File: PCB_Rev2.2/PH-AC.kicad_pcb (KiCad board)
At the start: 2 copper layers, 200 x 100 mm, 51 parts, among them J1 USB_C_Receptacle_USB2.0_16P, J2 Conn_01x03, SW1 SW_Push, SW10 SW_Push, SW2 RotaryEncoder_Switch_MP, SW3 RotaryEncoder_Switch_MP, SW4 SW_Push, SW5 SW_Push, SW6 SW_Push, SW7 SW_Push, SW8 SW_Push, SW9 SW_Push, U1 RP2040, U2 AMS1117-3.3, U3 W25Q16JVSS, Y1 Crystal_GND24

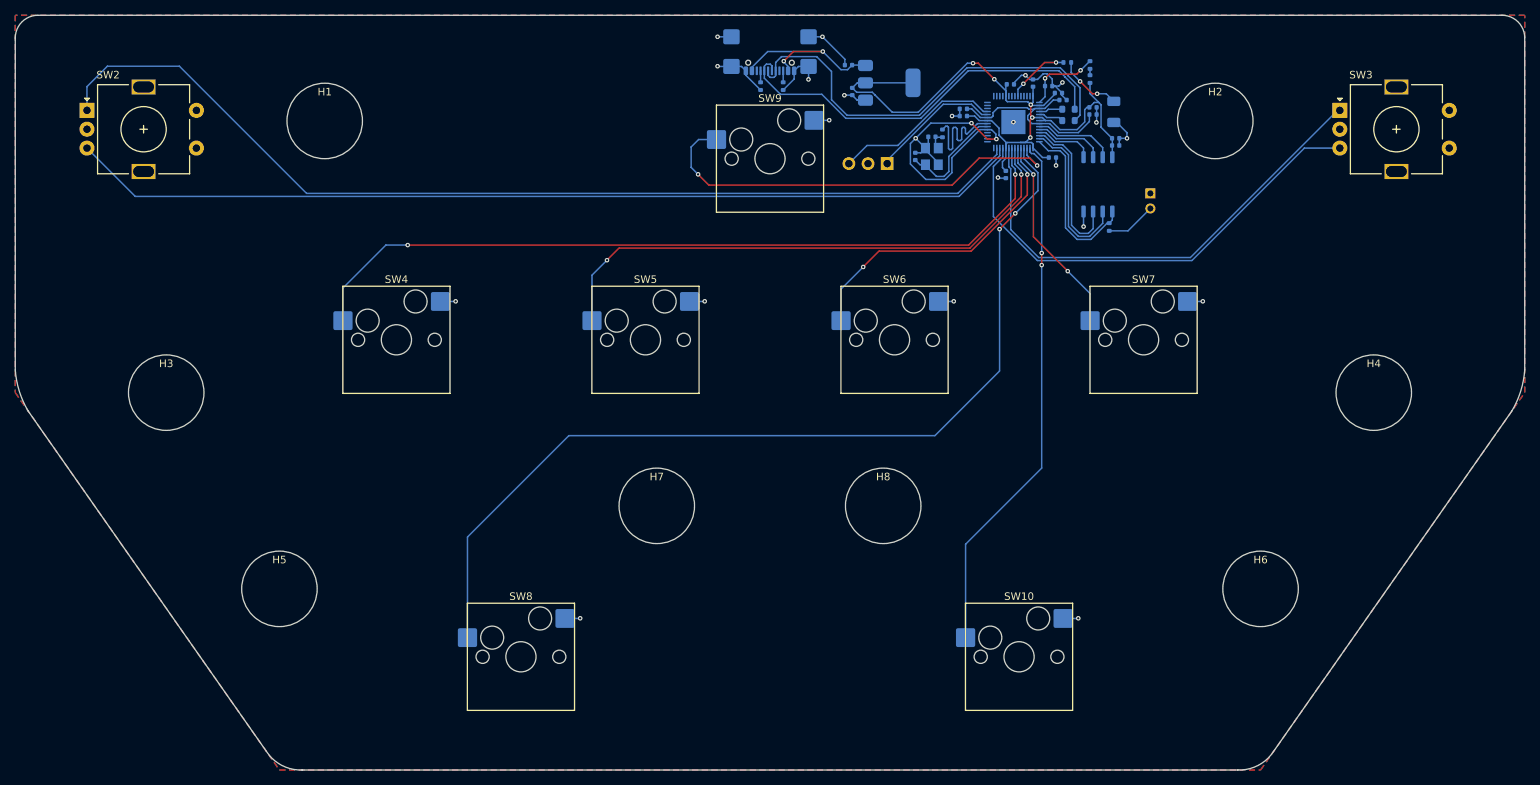
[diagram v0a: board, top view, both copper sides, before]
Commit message: Redesign
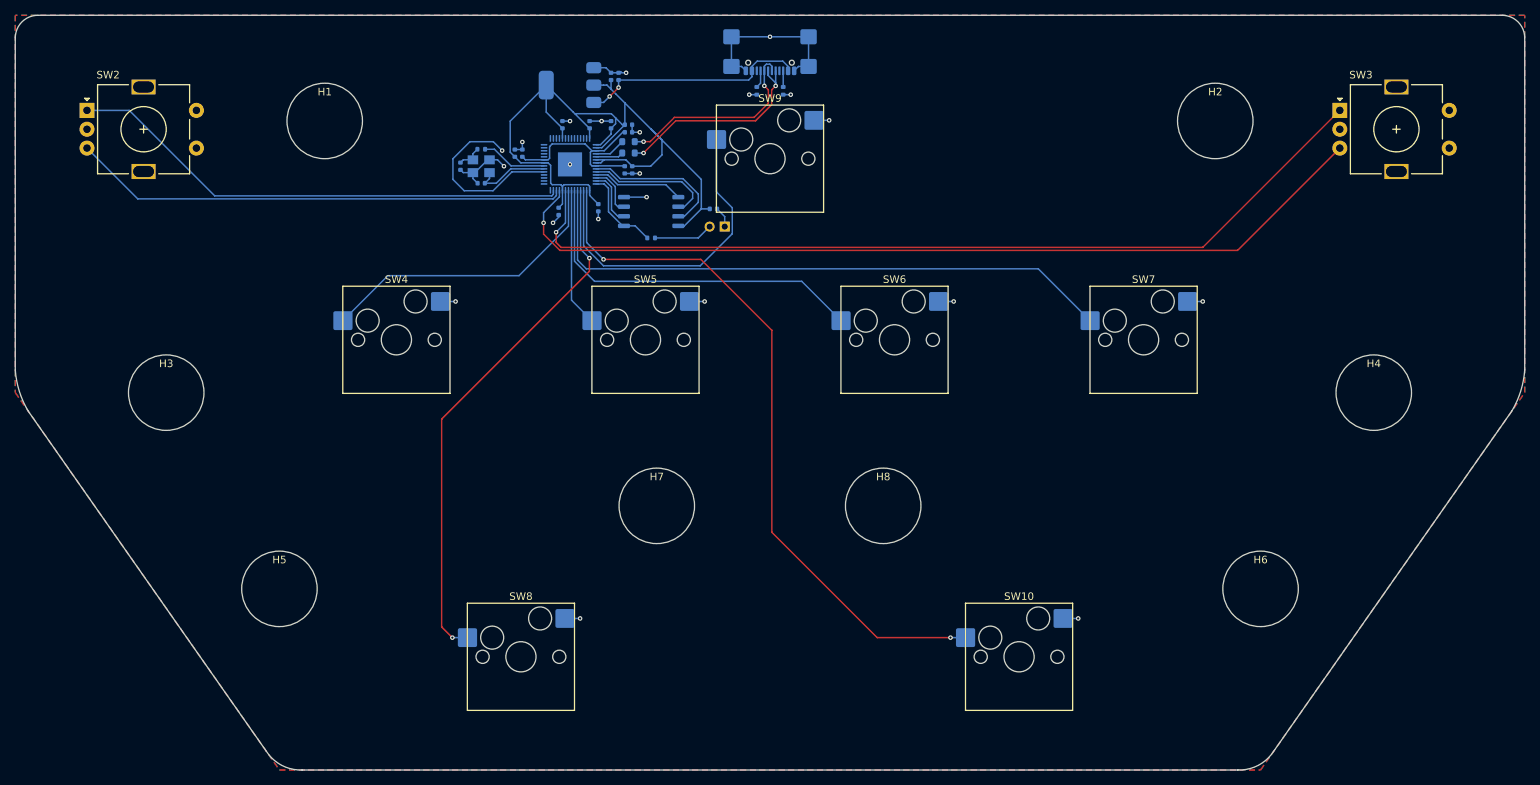
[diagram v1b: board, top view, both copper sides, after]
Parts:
- removed C17, C18: 20p, Capacitor_SMD:C_0402_1005Metric
- removed D2: LED, LED_SMD:LED_1206_3216Metric
- removed J2: Conn_01x03, Connector_PinHeader_2.54mm:PinHeader_1x03_P2.54mm_Vertical
- removed R12, R9: 1K, Resistor_SMD:R_0402_1005Metric
- removed R13: 470R, Resistor_SMD:R_0402_1005Metric
- removed R14, R15: 5K1, Resistor_SMD:R_0402_1005Metric
- removed R2: 200R, Resistor_SMD:R_0402_1005Metric
- added C16: 100n, Capacitor_SMD:C_0402_1005Metric, B.Cu at (146.4, 67.5)
- added R5: 1K, Resistor_SMD:R_0402_1005Metric, B.Cu at (129.2, 70.8)
- added R6: 5K1, Resistor_SMD:R_0402_1005Metric, B.Cu at (165.8, 63.0)
- added R7: 5K1, Resistor_SMD:R_0402_1005Metric, B.Cu at (169.2, 63.0)
- C1, C4: value 100n -> 10u
- C10: value 2u2 -> 1u
- C11, C14, C9: value 2u2 -> 100n
- C12, C13: value 10u -> 100n
- C2, C3: value 100n -> 20p
- C8: value 100n -> 1u
- R1: value 1R -> 1K
- moved C2 81.7 mm to (129.2, 75.2), turned to 180 degrees
- moved C7 75.8 mm to (134.7, 71.3), turned to 90 degrees
- moved C15 74.3 mm to (139.5, 79.0), turned to -90 degrees
- moved C14 69.2 mm to (144.8, 78.5), turned to -90 degrees
- moved C3 67.0 mm to (126.5, 73.0), turned to -90 degrees
- moved R1 62.5 mm to (151.8, 82.5), turned to 180 degrees
- moved C11 61.0 mm to (143.6, 67.5), turned to 90 degrees
- moved Y1 59.7 mm to (129.2, 73.0), turned to 180 degrees
- moved C4 59.5 mm to (146.4, 61.1), turned to 90 degrees
- moved U3 59.3 mm to (151.8, 79.0), turned to 0 degrees
- moved U1 59.0 mm to (141.0, 72.8)
- moved R3 58.5 mm to (148.8, 71.2)
- moved R4 58.5 mm to (148.8, 69.8)
- moved C9 57.8 mm to (149.2, 73.5), turned to -90 degrees
- moved C10 57.1 mm to (148.8, 67.5)
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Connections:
- net /USB_DM renamed /USB_DN
- C1 pad 1: +3V3 -> VBUS
- C11 pad 1: Net-(U1-ADC_AVDD) -> +3V3
- C12 pad 1: VBUS -> +3V3
- C2 pad 1: +3V3 -> /XIN
- C3 pad 1: +3V3 -> Net-(C3-Pad1)
- C6 pad 1: +3V3 -> +1V1
- C9 pad 1: +1V1 -> +3V3
- R1 pad 2: Net-(U1-ADC_AVDD) -> /QSPI_SS
- SW1 pad 2: Net-(R9-Pad1) -> Net-(R1-Pad1)
- U1 pad 24: Net-(J2-Pin_1) -> unconnected-(U1-SWCLK-Pad24)
- U1 pad 25: Net-(J2-Pin_3) -> unconnected-(U1-SWD-Pad25)
- U1 pad 37: Net-(U1-GPIO25) -> unconnected-(U1-GPIO25-Pad37)
- U1 pad 43: Net-(U1-ADC_AVDD) -> +3V3
- Y1 pad 3: Net-(C18-Pad1) -> Net-(C3-Pad1)
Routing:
- net ENC2A: track 134.8 -> 67.1 mm
- net BT0: track 105.3 -> 39.8 mm, vias 2 -> 0
- net ENC2B: track 126.9 -> 65.9 mm
- net BT1: track 74.1 -> 18.4 mm, vias 2 -> 0
- net BT4: track 125.5 -> 70.5 mm
- net ENC1A: track 64.1 -> 119.1 mm, vias 0 -> 1
- net ENC1B: track 64.1 -> 118.7 mm, vias 0 -> 1
- net BT3: track 26.8 -> 80.5 mm, vias 2 -> 0
- net /USB_DP: track 58.0 -> 27.9 mm, vias 0 -> 2
- net /USB_DN: track 53.9 -> 26.8 mm, vias 0 -> 2
- net BT6: track 70.0 -> 94.5 mm
- net Net-(J2-Pin_3): track 22.3 -> 0.00 mm
- net Net-(J2-Pin_1): track 17.4 -> 0.00 mm
- net +3V3: track 95.8 -> 112.9 mm, vias 5 -> 0
- net BT5: track 58.2 -> 43.3 mm, vias 2 -> 0
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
